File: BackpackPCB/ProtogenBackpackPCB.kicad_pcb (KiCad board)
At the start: 2 copper layers, 50 x 149.9 mm, 28 parts, among them J1 Pololu D24V10F3, J2 Pololu D36V28F5, J3 0.1" Header, J4 JST B6B-PH-K-S, J5 JST B6B-PH-K-S, J6 XLR5, M1 Conn_01x04_Male, M2 Conn_01x04_Male, SW1 Power Switch, U1 Pico, U2 TMC2209_SILENTSTEPSTICK, U3 TMC2209_SILENTSTEPSTICK, U4 TLC59108xPW

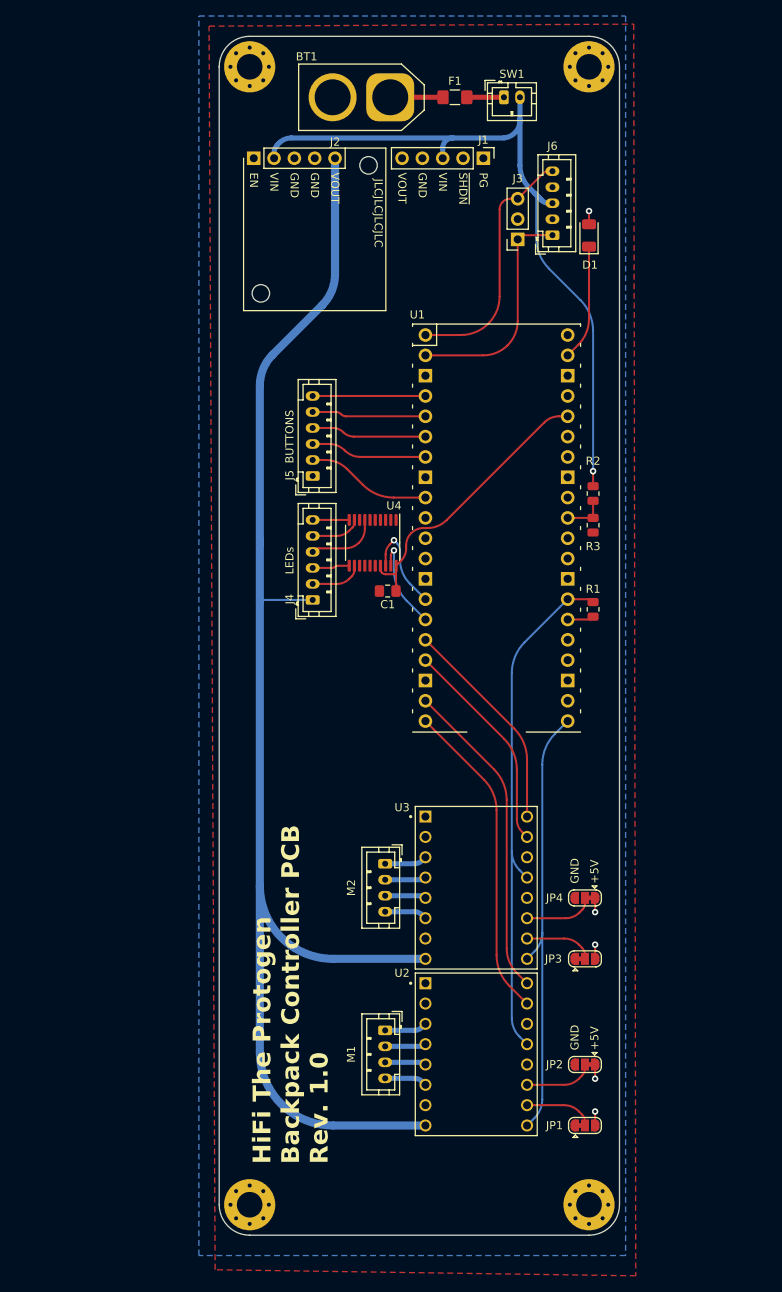
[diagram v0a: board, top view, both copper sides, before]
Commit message: Update to V2 of Backpack
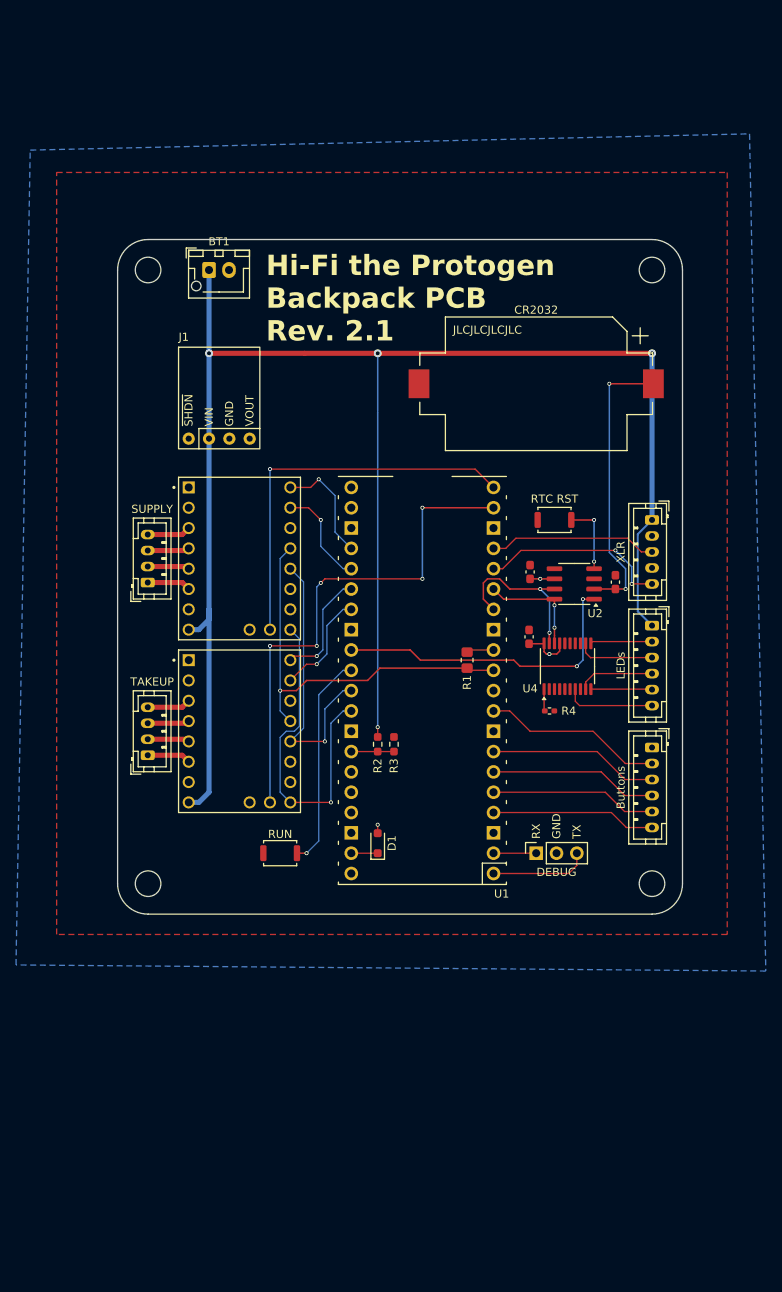
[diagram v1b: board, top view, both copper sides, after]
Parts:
- removed F1: Fuse, Fuse:Fuse_1206_3216Metric_Pad1.42x1.75mm_HandSolder
- removed J2: Pololu D36V28F5, MyloLibrary:Pololu D36V28Fx
- removed JP1, JP2, JP3, JP4: SolderJumper_3_Bridged12, Jumper:SolderJumper-3_P1.3mm_Bridged12_RoundedPad1.0x1.5mm
- removed U3: TMC2209_SILENTSTEPSTICK, TMC2209_SilentStepStick:MODULE_TMC2209_SILENTSTEPSTICK
- added BT2: CR2032, Battery:BatteryHolder_Keystone_1060_1x2032, F.Cu at (153.9, 68.8)
- added C2: 100 nF, Capacitor_SMD:C_0603_1608Metric_Pad1.08x0.95mm_HandSolder, F.Cu at (153.2, 92.4)
- added C3: 100 nF, Capacitor_SMD:C_0603_1608Metric_Pad1.08x0.95mm_HandSolder, F.Cu at (163.8, 93.6)
- added R4: 931Ω, Resistor_SMD:R_0402_1005Metric_Pad0.72x0.64mm_HandSolder, F.Cu at (155.6, 109.7)
- added SW2: SKRKAHE020, Button_Switch_SMD:SW_Push_SPST_NO_Alps_SKRK, F.Cu at (156.2, 85.9)
- added U5: TMC2209_SILENTSTEPSTICK, TMC2209 SilentStepStick:MODULE_TMC2209_SILENTSTEPSTICK, F.Cu at (116.8, 90.7)
- added U6: TMC2209_SILENTSTEPSTICK, TMC2209 SilentStepStick:MODULE_TMC2209_SILENTSTEPSTICK, F.Cu at (116.8, 112.3)
- BT1: value 10S Li-ion -> 3S Li-ion; footprint Connector_AMASS:AMASS_XT60-M_1x02_P7.20mm_Vertical -> Connector_JST:JST_XH_B2B-XH-AM_1x02_P2.50mm_Vertical
- C1: footprint Capacitor_SMD:C_0805_2012Metric_Pad1.18x1.45mm_HandSolder -> Capacitor_SMD:C_0603_1608Metric_Pad1.08x0.95mm_HandSolder
- D1: value ? -> SD103AWS; footprint Diode_SMD:D_1206_3216Metric -> Diode_SMD:D_SOD-323_HandSoldering
- H1, H2, H3, H4: footprint MountingHole:MountingHole_3.2mm_M3_Pad_Via -> MountingHole:MountingHole_3.2mm_M3_ISO7380
- J1: value Pololu D24V10F3 -> Pololu D24V5F3; footprint MyloLibrary:Pololu D24V10Fx -> TMC2209 SilentStepStick:Pololu_D24V5Fx
- R1: footprint Resistor_SMD:R_0805_2012Metric -> Resistor_SMD:R_0805_2012Metric_Pad1.20x1.40mm_HandSolder
- R2: value 11k -> 100k; footprint Resistor_SMD:R_0805_2012Metric -> Resistor_SMD:R_0603_1608Metric_Pad0.98x0.95mm_HandSolder
- R3: value 820 -> 30.1k; footprint Resistor_SMD:R_0805_2012Metric -> Resistor_SMD:R_0603_1608Metric_Pad0.98x0.95mm_HandSolder
- SW1: value Power Switch -> SKRKAHE020; footprint Connector_JST:JST_PH_B2B-PH-K_1x02_P2.00mm_Vertical -> Button_Switch_SMD:SW_Push_SPST_NO_Alps_SKRK
- U2: value TMC2209_SILENTSTEPSTICK -> DS3231MZ; footprint TMC2209_SilentStepStick:MODULE_TMC2209_SILENTSTEPSTICK -> Package_SO:SOIC-8_3.9x4.9mm_P1.27mm
- U4: value TLC59108xPW -> TLC59108FPW
- moved SW1 98.5 mm to (121.9, 127.5)
- moved D1 80.4 mm to (134.1, 126.3)
- moved J3 76.8 mm to (153.9, 127.5), turned to 90 degrees
- moved M1 63.4 mm to (105.4, 93.7), turned to 90 degrees
- moved U2 60.1 mm to (158.7, 93.9), turned to 180 degrees
- moved J5 54.3 mm to (168.4, 114.3), turned to -90 degrees
- moved J1 50.8 mm to (110.5, 75.7), turned to 0 degrees
- moved J4 42.5 mm to (168.4, 99.1), turned to -90 degrees
- moved H3 42.1 mm to (105.4, 131.3)
- moved R2 41.3 mm to (134.1, 113.9)
- moved H4 40.9 mm to (168.4, 131.3)
- moved J6 37.7 mm to (168.4, 85.9), turned to -90 degrees
- moved R3 37.0 mm to (136.1, 113.9), turned to 90 degrees
- moved M2 32.6 mm to (105.4, 115.3), turned to 90 degrees
- moved BT1 31.3 mm to (113.0, 54.6), turned to 0 degrees
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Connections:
- BT1 pad 1: Net-(BT1-+) -> +BATT
- D1 pad 2: VDD -> +3V3
- J1 pad 2: unconnected-(J1-~{SHDN}-Pad2) -> +BATT
- J1 pad 3: +BATT -> GND
- J1 pad 4: GND -> +3V3
- J3 pad 1: OUT_TX -> DBG_RX
- J3 pad 3: OUT_RX -> DBG_TX
- J4 pad 1: +12V -> +BATT
- J4 pad 2: Net-(J4-Pin_2) -> /LED4
- J4 pad 3: Net-(J4-Pin_3) -> /LED5
- J4 pad 4: Net-(J4-Pin_4) -> /LED2
- J4 pad 5: Net-(J4-Pin_5) -> /LED3
- J4 pad 6: Net-(J4-Pin_6) -> /LED1
- J5 pad 2: BUTTON_4 -> BUTTON_5
- J5 pad 3: BUTTON_3 -> BUTTON_4
- J5 pad 4: BUTTON_2 -> BUTTON_3
- J5 pad 5: BUTTON_1 -> BUTTON_2
- J5 pad 6: BUTTON_0 -> BUTTON_1
- J6 pad 1: OUT_TX -> +BATT
- J6 pad 3: +BATT -> OUT_RX
- J6 pad 5: OUT_RX -> OUT_TX
- M1 pad 1: M1A- -> M1B-
- M1 pad 2: M1A+ -> M1B+
- M1 pad 3: M1B+ -> M1A+
- M1 pad 4: M1B- -> M1A-
- M2 pad 1: M2A- -> M2B-
- M2 pad 2: M2A+ -> M2B+
- M2 pad 3: M2B+ -> M2A+
- M2 pad 4: M2B- -> M2A-
- R1 pad 2: Net-(U1-GPIO20) -> /S_TX
- SW1 pad 1: Net-(SW1-A) -> GND
- SW1 pad 2: +BATT -> RUN
- U1 pad 1: OUT_RX -> DBG_TX
- U1 pad 11: unconnected-(U1-GPIO8-Pad11) -> S_UART
- U1 pad 12: unconnected-(U1-GPIO9-Pad12) -> /S_TX
- U1 pad 14: LED_SDA -> SDA
- U1 pad 15: LED_SCL -> SCL
- U1 pad 16: BR_DIR -> OUT_TX
- U1 pad 17: BR_STEP -> OUT_RX
- U1 pad 19: TR_DIR -> BR_DIAG
- U1 pad 2: OUT_TX -> DBG_RX
- U1 pad 20: TR_STEP -> TR_DIAG
- U1 pad 21: REEL_~{EN} -> unconnected-(U1-GPIO16-Pad21)
- U1 pad 24: unconnected-(U1-GPIO18-Pad24) -> TR_DIR
- U1 pad 25: unconnected-(U1-GPIO19-Pad25) -> TR_STEP
- U1 pad 26: Net-(U1-GPIO20) -> BR_DIR
- U1 pad 27: S_UART -> BR_STEP
- U1 pad 29: unconnected-(U1-GPIO22-Pad29) -> 32KHz
- U1 pad 30: unconnected-(U1-RUN-Pad30) -> RUN
- U1 pad 31: BAT_VOLTAGE -> SPRD
- U1 pad 32: GND -> REEL_~{EN}
- U1 pad 34: unconnected-(U1-GPIO28_ADC2-Pad34) -> BAT_VOLTAGE
- U1 pad 36: +3V3 -> unconnected-(U1-3V3-Pad36)
- U1 pad 4: BUTTON_0 -> BUTTON_1
- U1 pad 5: BUTTON_1 -> BUTTON_2
- U1 pad 6: BUTTON_2 -> BUTTON_3
- U1 pad 7: BUTTON_3 -> BUTTON_4
- U1 pad 9: BUTTON_4 -> BUTTON_5
- U2 pad 1: GND -> 32KHz
- U2 pad 2: VDD -> Net-(BT2-+)
- U2 pad 3: M1A- -> unconnected-(U2-~{INT}/SQW-Pad3)
- U2 pad 4: M1A+ -> /~{RST}
- U2 pad 5: M1B+ -> GND
- U2 pad 6: M1B- -> +3V3
- U2 pad 7: GND -> SDA
- U2 pad 8: +12V -> SCL
- U4 pad 1: unconnected-(U4-REXT-Pad1) -> Net-(U4-REXT)
- U4 pad 10: Net-(J4-Pin_6) -> /LED3
- U4 pad 11: Net-(J4-Pin_3) -> /LED4
- U4 pad 12: Net-(J4-Pin_2) -> /LED5
- U4 pad 18: LED_SDA -> SCL
- U4 pad 19: LED_SCL -> SDA
- U4 pad 7: Net-(J4-Pin_4) -> /LED1
- U4 pad 9: Net-(J4-Pin_5) -> /LED2
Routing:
- net +12V: track 173.4 -> 0.00 mm
- net +BATT: track 90.5 -> 211.5 mm, vias 1 -> 4
- net BR_DIAG: track 0.00 -> 64.2 mm, vias 0 -> 5
- net TR_DIAG: track 0.00 -> 49.0 mm, vias 0 -> 1
- net 32KHz: track 0.00 -> 39.2 mm, vias 0 -> 2
- net Net-(BT2-+): track 0.00 -> 35.9 mm, vias 0 -> 2
- net SPRD: track 0.00 -> 35.6 mm, vias 0 -> 1
- net TR_STEP: track 40.0 -> 12.7 mm, vias 0 -> 1
- net RUN: track 0.00 -> 27.0 mm, vias 0 -> 1
- net +3V3: track 36.3 -> 10.2 mm, vias 0 -> 3
- net TR_DIR: track 40.1 -> 14.3 mm, vias 0 -> 1
- net BUTTON_5: track 0.00 -> 22.5 mm
- net SDA: track 0.00 -> 20.8 mm, vias 0 -> 2
- net S_UART: track 65.6 -> 50.6 mm, vias 0 -> 1
- net BUTTON_0: track 14.1 -> 0.00 mm
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- added copper zone on B.Cu, net +3V3
- removed copper zone on B.Cu, net VDD
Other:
- board size 50 x 149.9 mm -> 70.6 x 84.3 mm
- board text added: "+BATT"
- board text added: "BTN1"
- board text added: "BTN2"
- board text added: "BTN3"
- board text added: "BTN4"
- board text added: "BTN5"
- board text added: "Buttons"
- board text added: "CR2032"
- board text added: "DEBUG"
- board text added: "Hi-Fi the Protogen Backpack PCB Rev. 2.1"
- board text added: "LED1"
- board text added: "LED2"
- board text added: "LED3"
- board text added: "LED4"
- board text added: "LED5"
- board text added: "RTC RST"
- board text added: "RUN"
- board text added: "RX"
- board text added: "SUPPLY"
- board text added: "TAKEUP"
- board text added: "TX"
- board text added: "XLR"
- board text removed: "+5V"
- board text removed: "BUTTONS"
- board text removed: "HiFi The Protogen Backpack Controller PCB Rev. 1.0"
